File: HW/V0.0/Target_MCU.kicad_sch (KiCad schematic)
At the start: 25 parts, among them J3 EXP PORT, SW1 UBT, U10 20MHz, U4 PIC16F877A

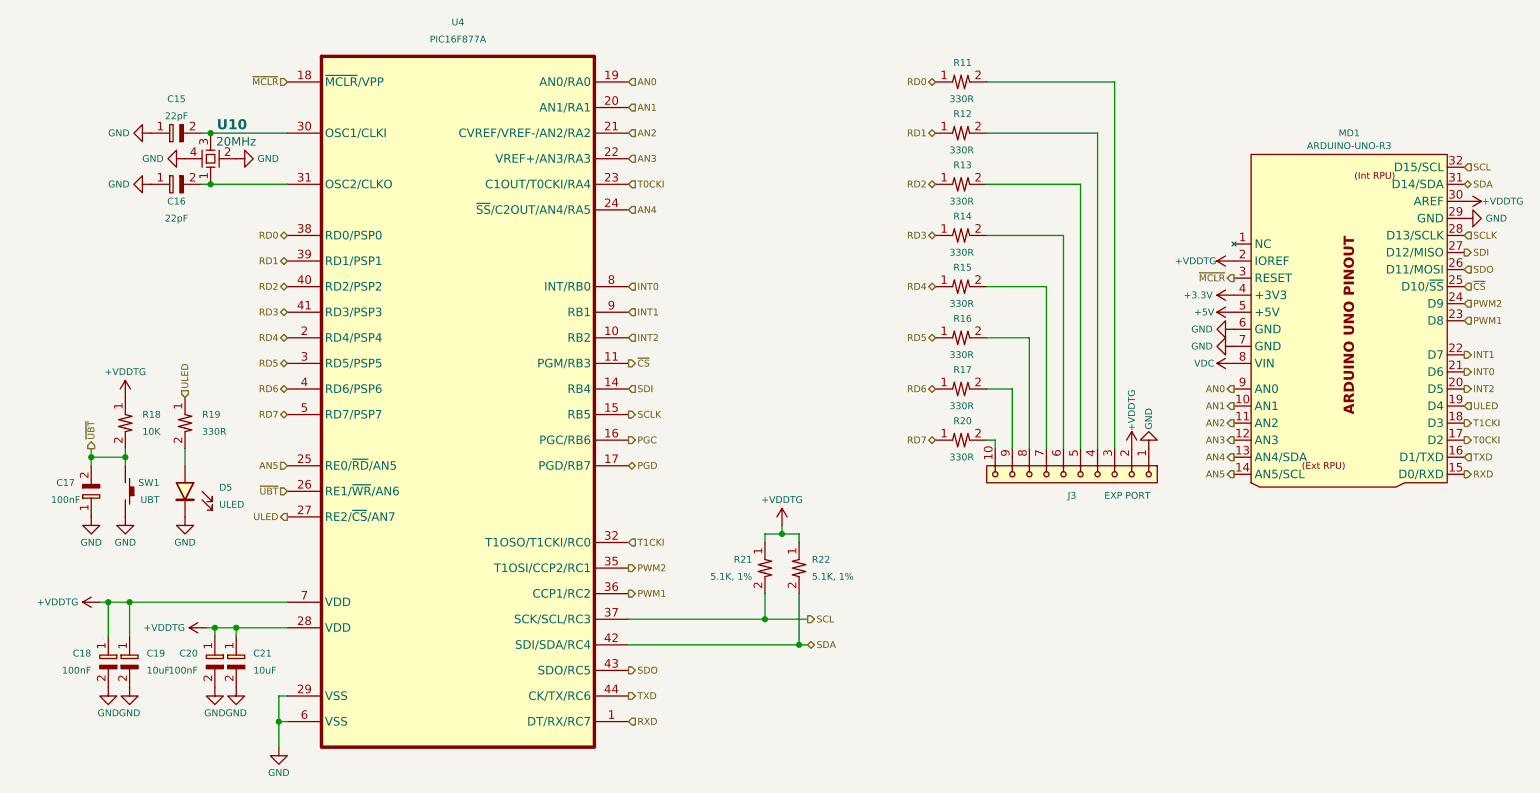
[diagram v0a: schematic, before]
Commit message: PIC16-DevKit-SCH-877 schematic update 6
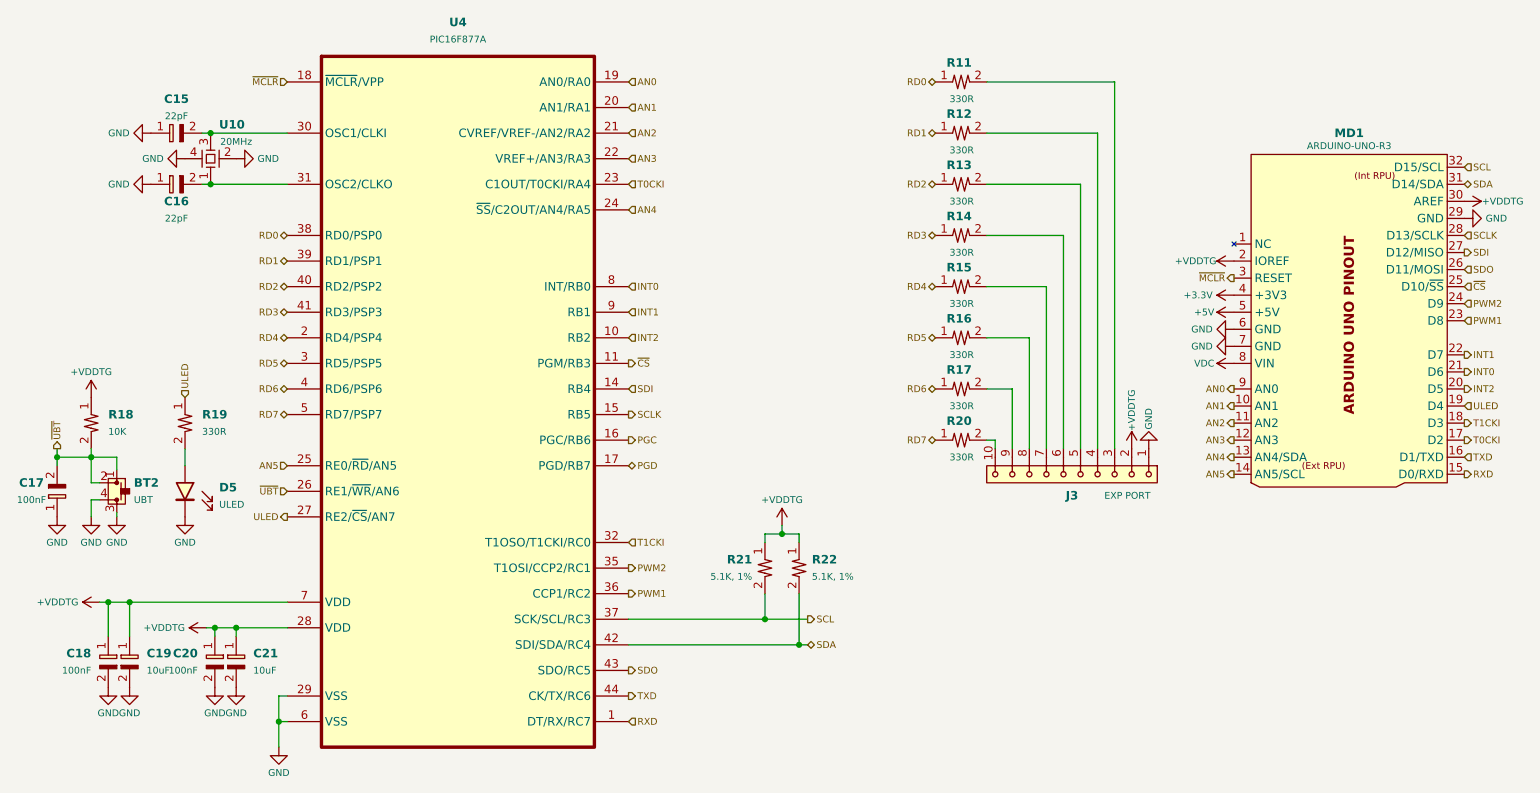
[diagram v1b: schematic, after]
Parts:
- removed SW1: UBT, Triet_KiCAD_Fprint:SW_2P_3.5x6, symbol Triet_KiCAD_Sym:Switch_2P
- added BT2: UBT, Liem:SW6x6-G, symbol SAMPI:BT2
- C15, C16: MFT (none) -> Walsin; MNP (none) -> 0603N220J500CT
- C17, C18, C20: MFT (none) -> Samsung; MNP (none) -> CL10B104KB8NNNC
- C19, C21: MFT (none) -> Samsung; MNP (none) -> CL10A106MQ8NNNC
- D5: MFT (none) -> Harvatek; MNP (none) -> B1911NG--20D000214U1930
- J3: footprint SAMPI:HDM1x10x2.54_TH_RA -> SAMPI:HDM1x10x2.54_TH; MFT (none) -> Adam Tech; MNP (none) -> RS1-10-G
- MD1: MFT (none) -> JLCPCB; MNP (none) -> PCB.SAMM-877A
- R11, R12, R13, R14, R15, R16, R17, R19, R20: MFT (none) -> Yageo; MNP (none) -> RC0603JR-07330RL
- R18: MFT (none) -> Yageo; MNP (none) -> RC0603JR-0710KL
- R21, R22: MFT (none) -> Yageo; MNP (none) -> RC0603FR-075K1L
- U10: MFT (none) -> Diodes; MNP (none) -> FL2000038
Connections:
- net GND: now also BT2.3, BT2.4
- net ~{UBT}: now also BT2.1, BT2.2
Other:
- moved on the sheet: C17, R18
